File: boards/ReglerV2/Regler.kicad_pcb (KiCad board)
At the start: 2 copper layers, 160 x 50 mm, 18 parts, among them J1 In_L, J2 In_R, J3 12V_In, J4 Switch, J5 Out_L, J6 Out_R, K1 DIPxx-2Axx-21x, K2 DIPxx-2Axx-21x, K3 DIPxx-2Axx-21x, K4 DIPxx-2Axx-21x

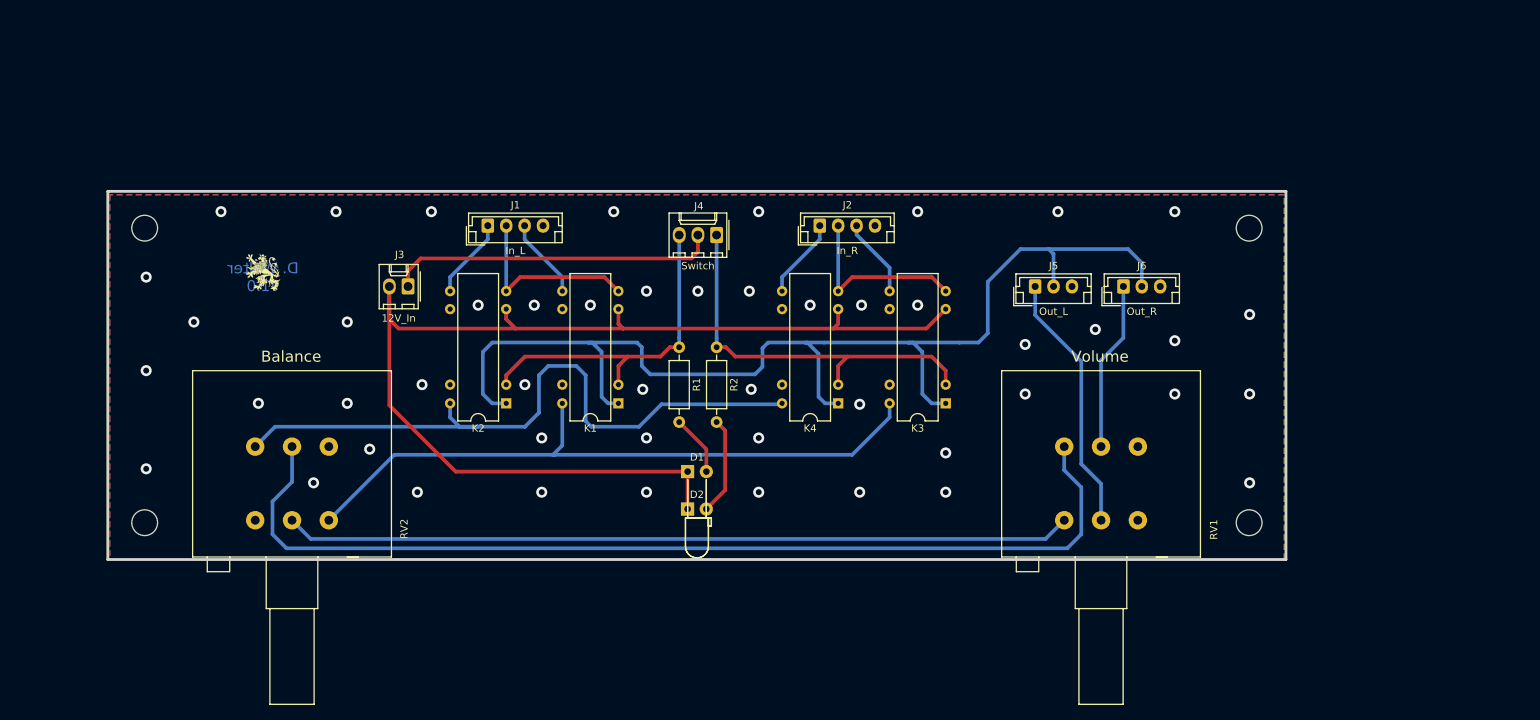
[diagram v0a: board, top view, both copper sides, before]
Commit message: Work in progess - many LAyour changes
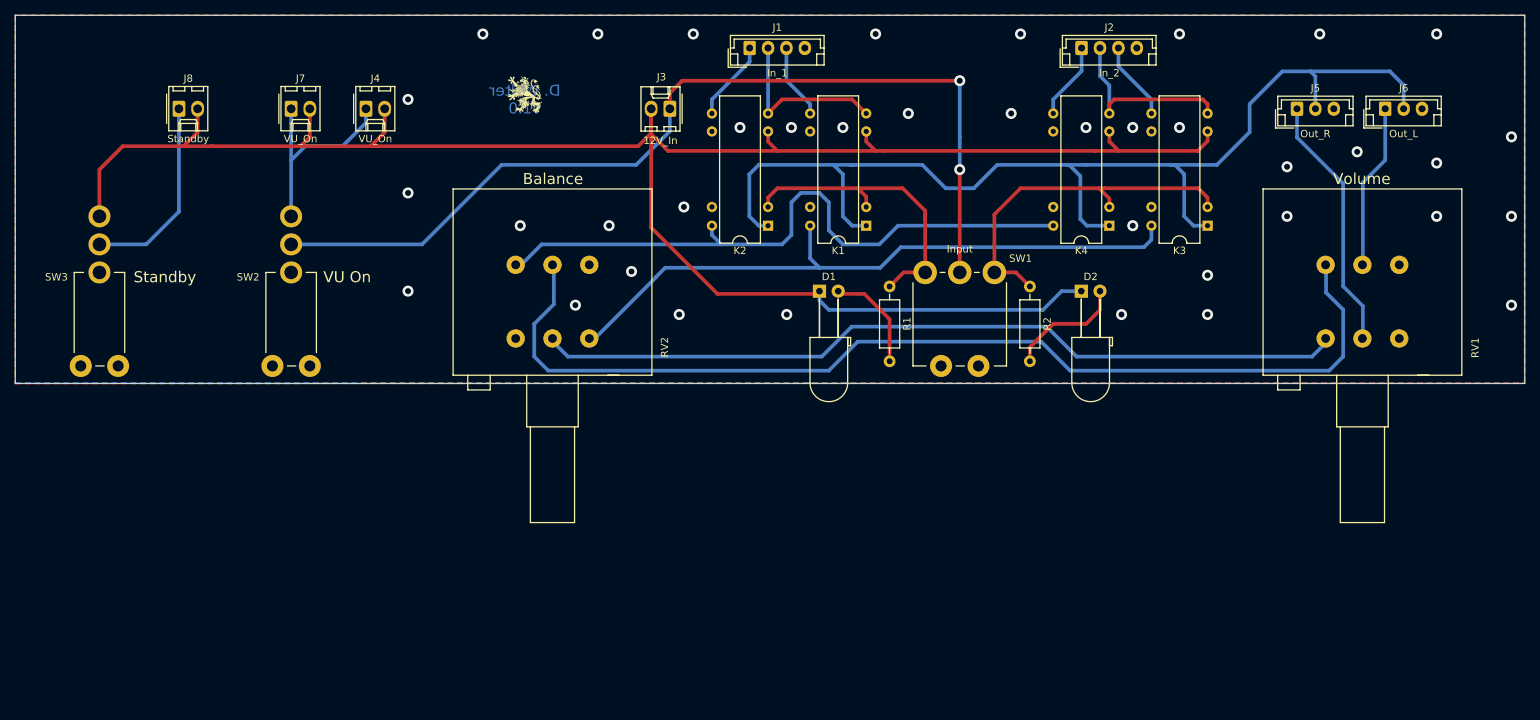
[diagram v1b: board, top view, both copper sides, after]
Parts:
- removed REF**: EuroBoard_halb_Type-II_160mmX50mm_holes, EuroBoard_Outline:EuroBoard_halb_Type-II_160mmX50mm_holes
- added J7: VU_On, Connector_Molex:Molex_KK-254_AE-6410-02A_1x02_P2.54mm_Vertical, F.Cu at (78.7, 76.2)
- added J8: Standby, Connector_Molex:Molex_KK-254_AE-6410-02A_1x02_P2.54mm_Vertical, F.Cu at (63.5, 76.2)
- added SW1: Input, Switch_Angled:7101MD9ABE, F.Cu at (169.5, 98.4)
- added SW2: VU_On, Switch_Angled:7101MD9AV2BE, F.Cu at (78.7, 94.6)
- added SW3: Standby, Switch_Angled:7101MD9AV2BE, F.Cu at (52.7, 94.6)
- D1: footprint LED_THT:LED_D3.0mm_Horizontal_O6.35mm_Z6.0mm -> LED_THT:LED_D5.0mm_Horizontal_O6.35mm_Z9.0mm
- D2: footprint LED_THT:LED_D3.0mm_Horizontal_O1.27mm_Z6.0mm -> LED_THT:LED_D5.0mm_Horizontal_O6.35mm_Z9.0mm
- J1: value In_L -> In_1
- J2: value In_R -> In_2
- J4: value Switch -> VU_On; footprint Connector_Molex:Molex_KK-254_AE-6410-03A_1x03_P2.54mm_Vertical -> Connector_Molex:Molex_KK-254_AE-6410-02A_1x02_P2.54mm_Vertical
- J5: value Out_L -> Out_R
- J6: value Out_R -> Out_L
- moved D2 61.1 mm to (186.1, 101.0)
- moved J4 50.6 mm to (88.9, 76.2), turned to 0 degrees
- moved K4 44.0 mm to (189.9, 92.1)
- moved R2 43.3 mm to (179.1, 100.3)
- moved RV1 43.2 mm to (229.2, 108.6)
- moved RV2 43.1 mm to (119.2, 108.6)
- moved J3 43.0 mm to (130.2, 76.2)
- moved J2 43.0 mm to (186.1, 67.9)
- moved J1 43.0 mm to (141.0, 67.9)
- moved J5 43.0 mm to (215.3, 76.2)
- moved J6 43.0 mm to (227.3, 76.2)
- moved K3 43.0 mm to (203.2, 92.1)
- moved G*** 43.0 mm to (110.5, 74.3)
- moved K2 43.0 mm to (143.5, 92.1)
- moved K1 41.4 mm to (156.8, 92.1)
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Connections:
- J1 pad 1: /R_1 -> /L_1
- J1 pad 3: /L_1 -> /R_1
- J2 pad 1: /R_2 -> /L_2
- J2 pad 3: /L_2 -> /R_2
- J4 pad 1: /CH_2 -> Net-(J4-Pad1)
- J4 pad 2: +12V -> GND
- J5 pad 1: /L_Out -> /R_Out
- J6 pad 1: /R_Out -> /L_Out
- K1 pad 14: /L_Sw -> /R_Sw
- K1 pad 8: /L_1 -> /R_1
- K2 pad 14: /R_Sw -> /L_Sw
- K2 pad 8: /R_1 -> /L_1
- K3 pad 14: /L_Sw -> /R_Sw
- K3 pad 8: /L_2 -> /R_2
- K4 pad 14: /R_Sw -> /L_Sw
- K4 pad 8: /R_2 -> /L_2
- RV1 pad 2: /L_Out -> /R_Out
- RV1 pad 5: /R_Out -> /L_Out
- RV2 pad 3: /L_Sw -> /R_Sw
- RV2 pad 4: /R_Sw -> /L_Sw
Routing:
- net GND: track 156.1 -> 272.7 mm
- net +12V: track 44.8 -> 129.1 mm, vias 0 -> 2
- net Net-(J4-Pad1): track 0.00 -> 28.8 mm
- net Net-(J8-Pad1): track 0.00 -> 26.6 mm
- net /L_Out: track 35.5 -> 23.0 mm
- net /R_Out: track 23.0 -> 35.5 mm
- net Net-(D1-Pad2): track 8.26 -> 14.1 mm
- net GNDS: track 158.9 -> 153.8 mm
- net /CH_2: track 53.9 -> 48.8 mm
- net /CH_1: track 45.9 -> 42.0 mm
- net /R_Sw: track 93.7 -> 90.1 mm
- net Net-(RV1-Pad4): track 137.3 -> 140.6 mm
- net Net-(RV1-Pad1): track 107.1 -> 109.9 mm
- net Net-(D2-Pad2): track 13.3 -> 16.1 mm
- net /L_Sw: track 91.6 -> 88.9 mm
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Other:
- board size 160 x 50 mm -> 205 x 50 mm
- board text added: "Standby"
- board text added: "VU On"
